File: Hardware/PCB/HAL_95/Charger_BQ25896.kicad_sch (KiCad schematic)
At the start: 49 parts, among them J9 Battery, Q1 DMN313DLT-7, Q2 DMP1045U-7, Q3 MMDT2907A-7-F, SW3 nQON, U3 BU33SD5WG-TR, U5 BQ25896RTW, U8 BQ27220YZFR

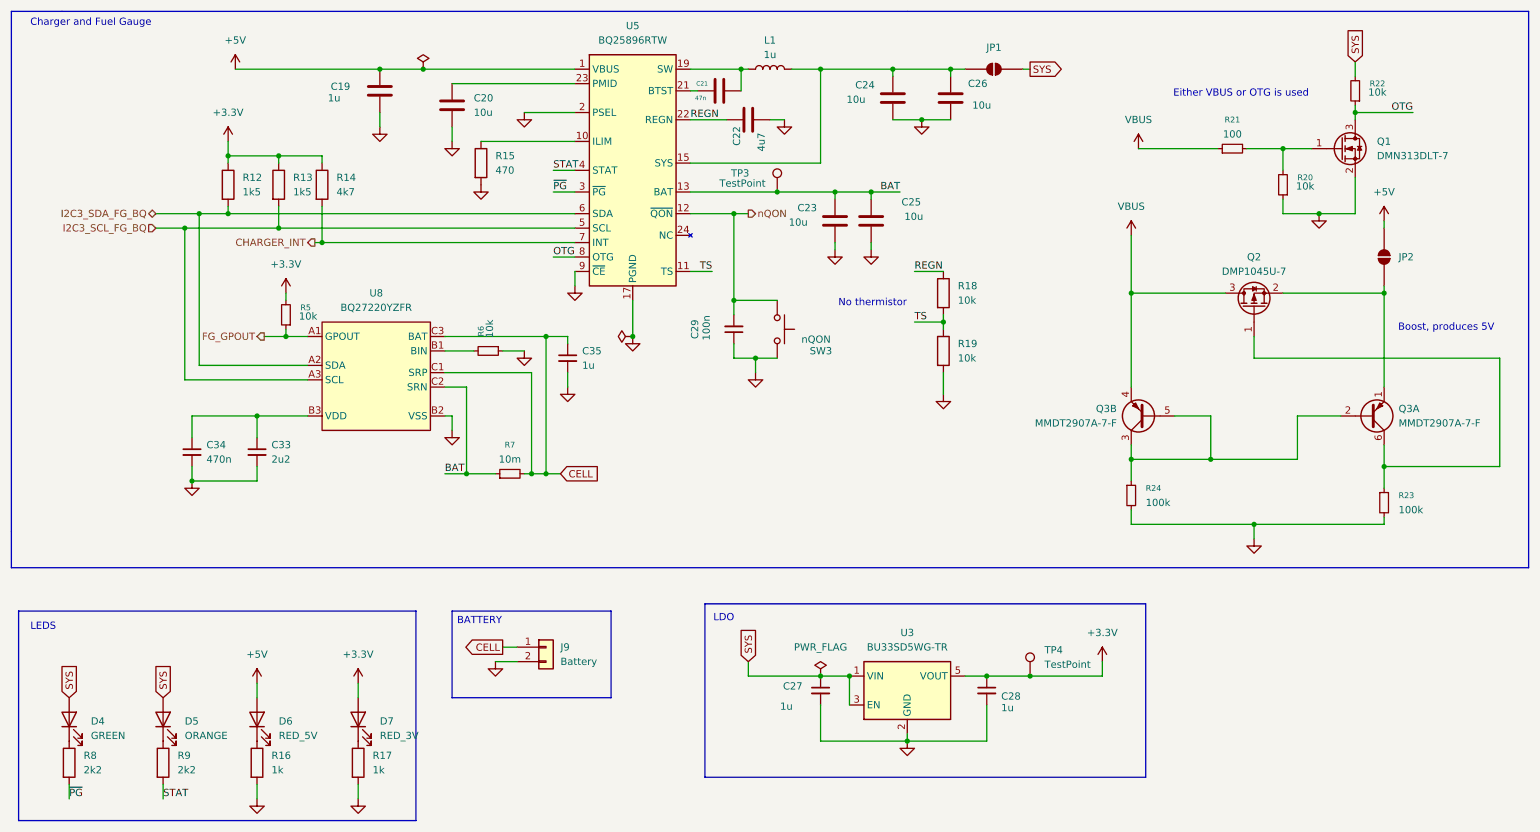
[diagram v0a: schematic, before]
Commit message: enhanced routing
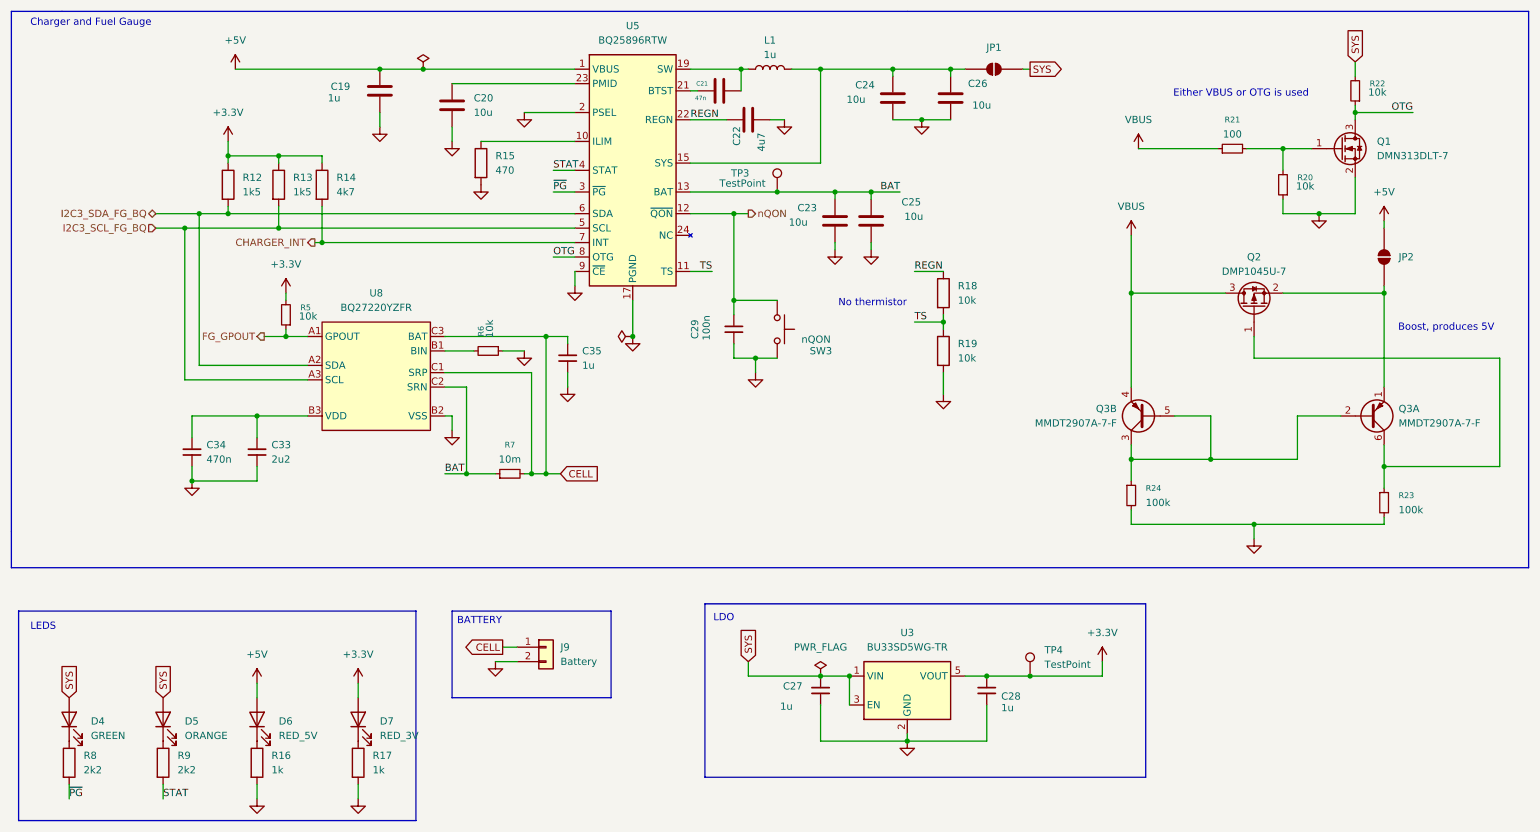
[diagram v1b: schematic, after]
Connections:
- net GND: now also U5.25 (PGND)
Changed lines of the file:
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@@
 		(pin "21"
+		)
+		(pin "25"
 		)
 		(instances

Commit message: added logo
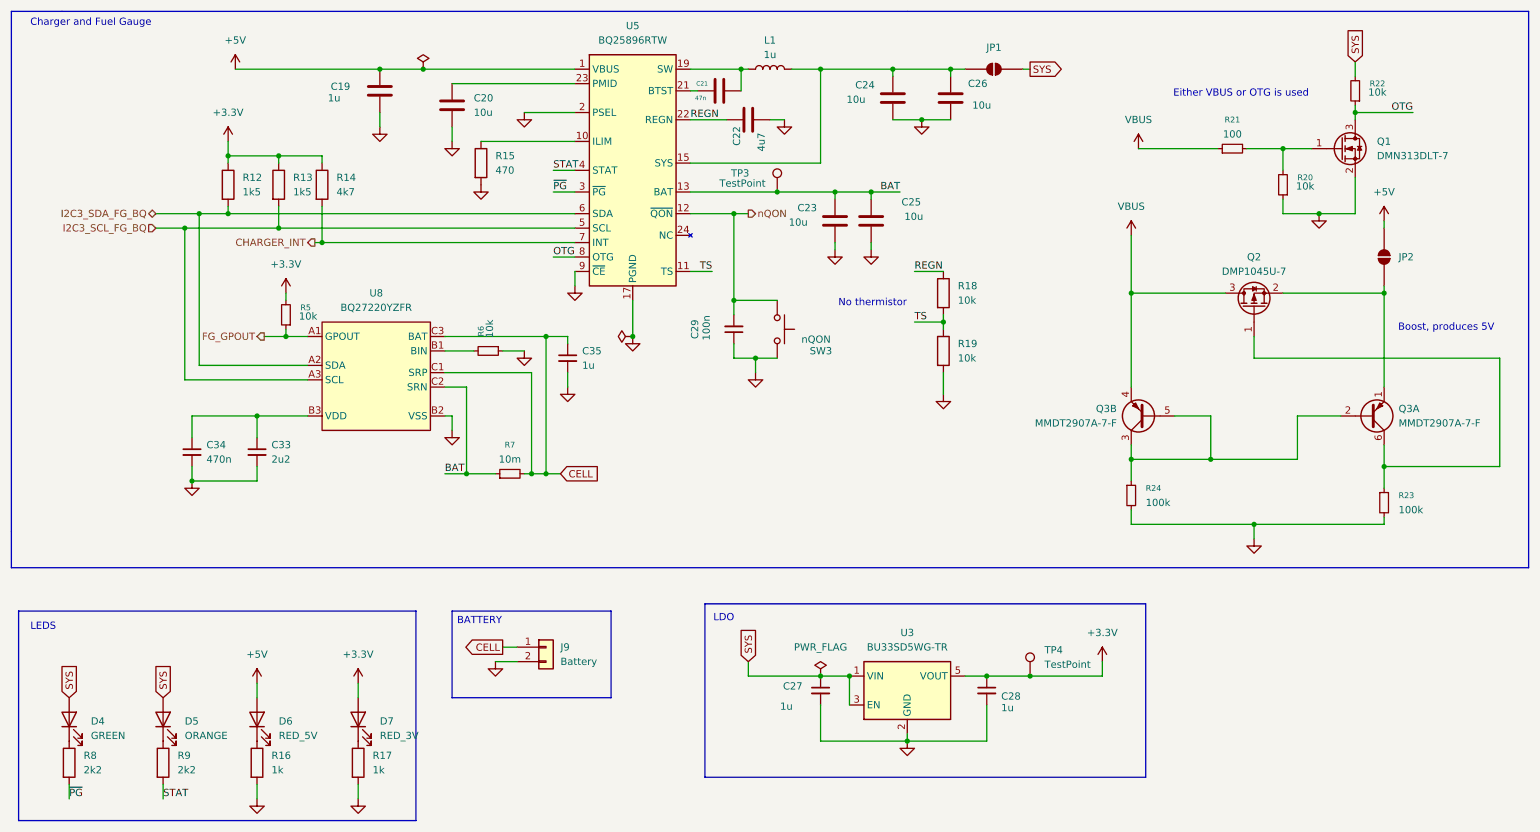
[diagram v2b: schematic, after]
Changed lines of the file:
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@@
+	)
+	(junction
+		(at 52.07 54.61)
+		(diameter 0)
+		(color 0 0 0 0)
 	)
 	(junction
@@
 	(junction
 		(at 193.04 135.89)
+		(diameter 0)
+		(color 0 0 0 0)
+	)
+	(junction
+		(at 140.97 54.61)
 		(diameter 0)
 		(color 0 0 0 0)
@@
 	)
 	(junction
-		(at 148.59 50.8)
-		(diameter 0)
-		(color 0 0 0 0)
-	)
-	(junction
 		(at 173.99 38.1)
 		(diameter 0)
@@
 	(junction
 		(at 57.15 90.17)
+		(diameter 0)
+		(color 0 0 0 0)
+	)
+	(junction
+		(at 68.58 59.69)
 		(diameter 0)
 		(color 0 0 0 0)
@@
 	)
 	(junction
-		(at 161.29 135.89)
+		(at 86.36 29.21)
 		(diameter 0)
 		(color 0 0 0 0)
@@
 	(junction
 		(at 123.19 76.2)
+		(diameter 0)
+		(color 0 0 0 0)
+	)
+	(junction
+		(at 161.29 135.89)
 		(diameter 0)
 		(color 0 0 0 0)
@@
 	)
 	(junction
-		(at 140.97 54.61)
+		(at 60.96 57.15)
 		(diameter 0)
 		(color 0 0 0 0)
@@
 	)
 	(junction
+		(at 148.59 50.8)
+		(diameter 0)
+		(color 0 0 0 0)
+	)
+	(junction
 		(at 232.41 109.22)
 		(diameter 0)
@@
 	)
 	(junction
-		(at 86.36 29.21)
-		(diameter 0)
-		(color 0 0 0 0)
-	)
-	(junction
 		(at 168.91 29.21)
-		(diameter 0)
-		(color 0 0 0 0)
-	)
-	(junction
-		(at 60.96 57.15)
-		(diameter 0)
-		(color 0 0 0 0)
-	)
-	(junction
-		(at 52.07 54.61)
 		(diameter 0)
 		(color 0 0 0 0)
@@
 		(diameter 0)
 		(color 0 0 0 0)
-	)
-	(junction
-		(at 68.58 59.69)
-		(diameter 0)
-		(color 0 0 0 0)
